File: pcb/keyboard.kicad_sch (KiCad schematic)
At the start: 27 parts, among them J1 Conn_ARM_JTAG_SWD_10, SW1 SW_Push, U1 nRF52840, X1 32MHz

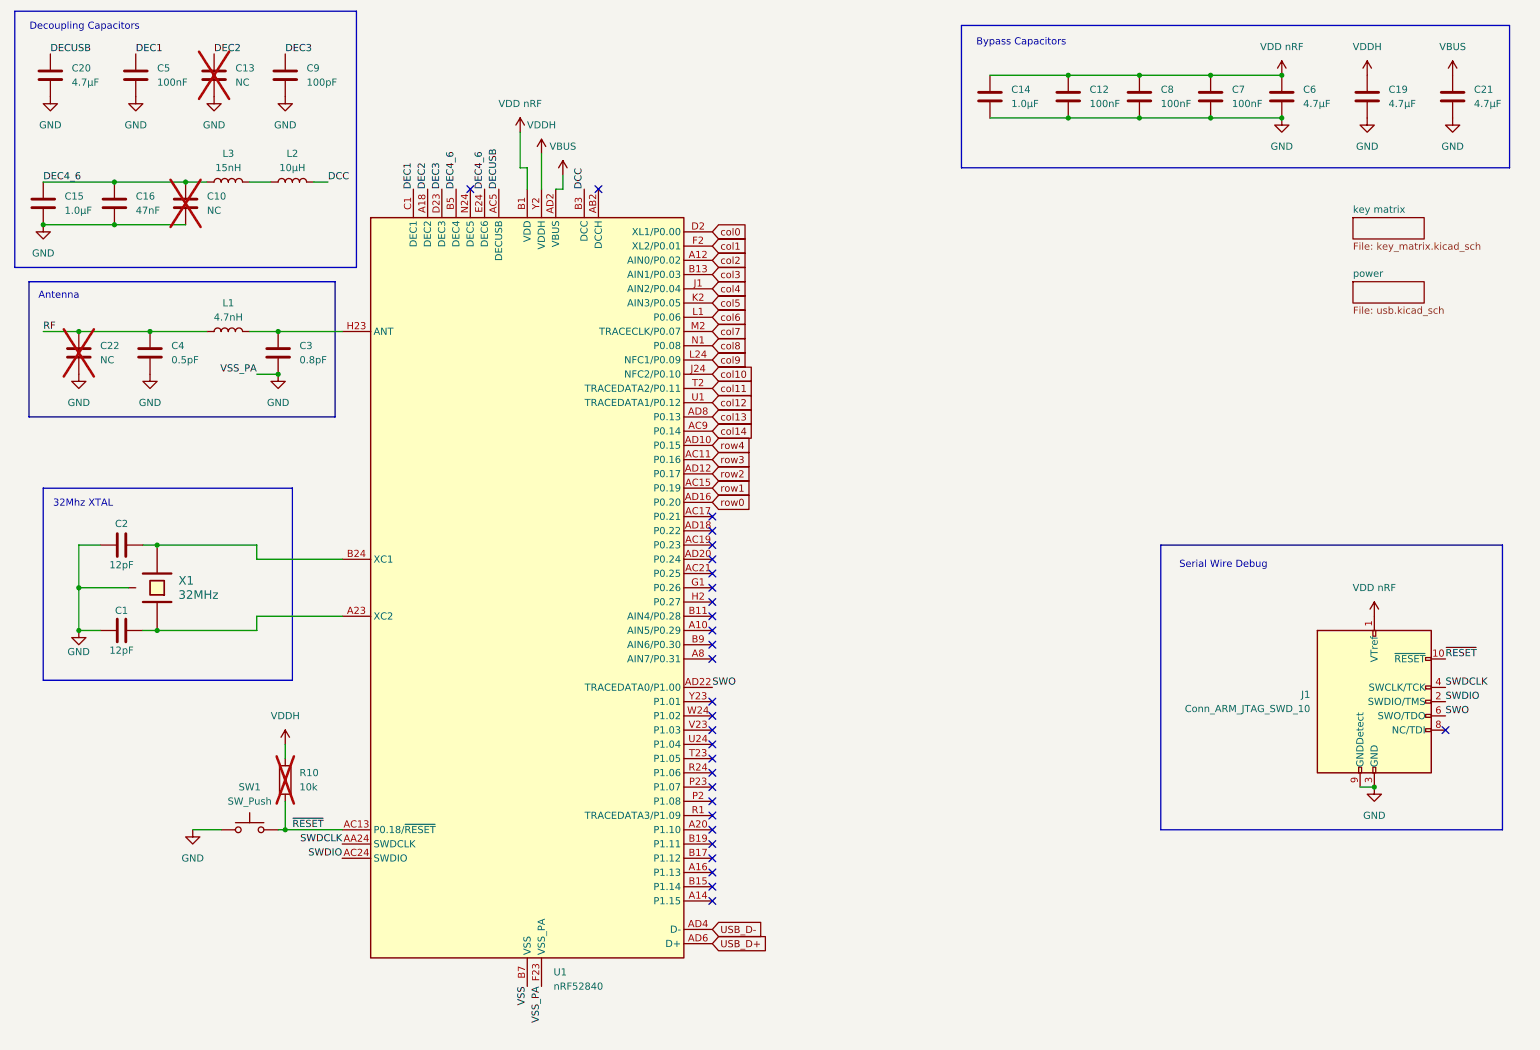
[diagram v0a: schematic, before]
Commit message: tinkering >:3
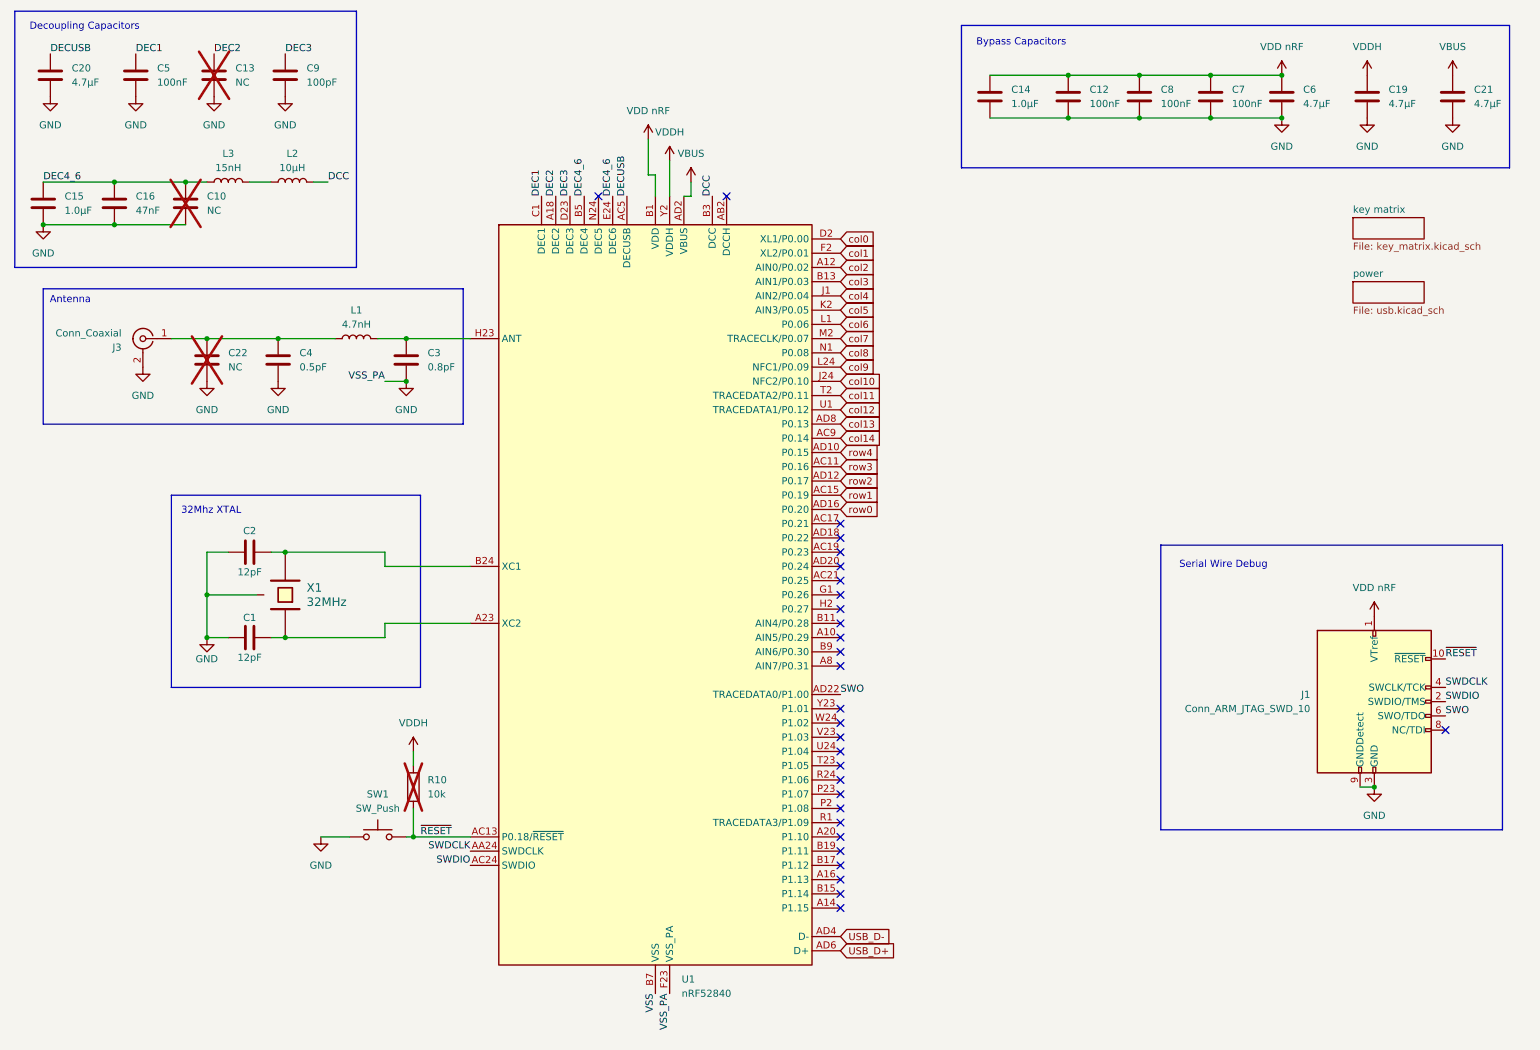
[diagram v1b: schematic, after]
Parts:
- added J3: Conn_Coaxial, Connector_Coaxial:SMA_Molex_73251-1153_EdgeMount_Horizontal, symbol Connector:Conn_Coaxial
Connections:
- net GND: now also J3.2 (Ext)
- net RF: no longer names the net of C22.1, C4.1, L1.1
- net RF: now also J3.1 (In)
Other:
- moved on the sheet: C1, C2, C22, C3, C4, L1, R10, SW1, U1, X1
